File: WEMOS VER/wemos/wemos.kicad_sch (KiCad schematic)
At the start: 15 parts, among them J1 9V BATT, J2 MOTOR 1, J3 MOTOR 2, SW1 RESET, SW2 ON/OFF, U1 WeMos D1 Mini, U2 L7805, U3 L293D

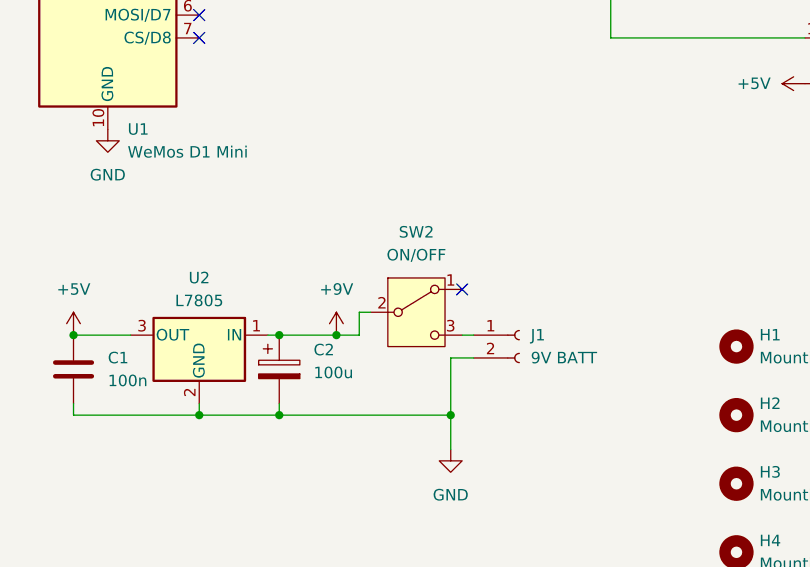
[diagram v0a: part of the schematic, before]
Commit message: revisions
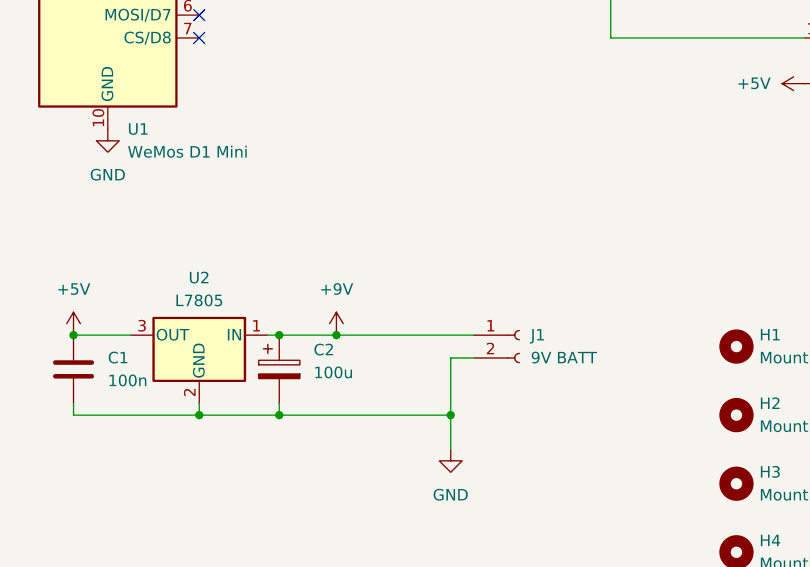
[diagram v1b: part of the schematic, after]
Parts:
- removed SW2: ON/OFF, Connector_PinSocket_2.54mm:PinSocket_1x03_P2.54mm_Vertical, symbol Switch:SW_SPDT
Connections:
- net +9V: now also J1.1 (Pin_1)
- no-connect marks 9 -> 8
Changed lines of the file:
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@@
-	)
-	(no_connect
-		(at 125.73 101.6)
 	)
 	(no_connect
@@
 	(wire
 		(pts
-			(xy 114.3 104.14) (xy 115.57 104.14)
-		)
-		(stroke
-			(width 0)
-			(type default)
-		)
-	)
-	(wire
-		(pts
-			(xy 114.3 104.14) (xy 114.3 106.68)
-		)
-		(stroke
-			(width 0)
-			(type default)
-		)
-	)
-	(wire
-		(pts
 			(xy 82.55 114.3) (xy 82.55 115.57)
 		)
@@
 	(wire
 		(pts
-			(xy 125.73 106.68) (xy 127 106.68)
+			(xy 111.76 106.68) (xy 127 106.68)
 		)
 		(stroke
@@
 		(pts
 			(xy 179.07 90.17) (xy 173.99 90.17)
-		)
-		(stroke
-			(width 0)
-			(type default)
-		)
-	)
-	(wire
-		(pts
-			(xy 111.76 106.68) (xy 114.3 106.68)
 		)
 		(stroke
@@
 					(unit 1)
 				)
-			)
-		)
-	)
-	(symbol
-		(lib_id "Switch:SW_SPDT")
-		(at 120.65 104.14 0)
-		(unit 1)
-		(exclude_from_sim no)
-		(in_bom yes)
-		(on_board yes)
-		(dnp no)
-		(fields_autoplaced yes)
-		(property "Reference" "SW2"
-			(at 120.65 95.25 0)
-			(effects
-				(font
-					(size 1.27 1.27)
-				)
-			)
-		)
-		(property "Value" "ON/OFF"
-			(at 120.65 97.79 0)
-			(effects
-				(font
-					(size 1.27 1.27)
-				)
-			)
-		)
-		(property "Footprint" "Connector_PinSocket_2.54mm:PinSocket_1x03_P2.54mm_Vertical"
-			(at 120.65 104.14 0)
-			(effects
-				(font
-					(size 1.27 1.27)
-				)
-				(hide yes)
-			)
-		)
-		(property "Datasheet" "~"
-			(at 120.65 111.76 0)
-			(effects
-				(font
-					(size 1.27 1.27)
-				)
-				(hide yes)
-			)
-		)
-		(property "Description" "Switch, single pole double throw"
-			(at 120.65 104.14 0)
-			(effects
-				(font
-					(size 1.27 1.27)
-				)
-				(hide yes)
-			)
-		)
-		(pin "3"
-		)
-		(pin "2"
-		)
-		(pin "1"
-		)
-		(instances
-			(project "wemos"
-				(path "/2ce77040-cfc1-475e-b4fd-779c85eca747"
-					(reference "SW2")
-					(unit 1)
-				)
